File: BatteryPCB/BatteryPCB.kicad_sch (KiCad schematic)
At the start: 18 parts, among them J1 Conn_01x01, J2 Conn_01x01, J3 Conn_01x01, J4 Conn_01x01_Socket, SW1 ANT11TFHQE, SW3 ANT11TFHQE, U1 LF50CV, U2 R05-100B, U3 R05-100B

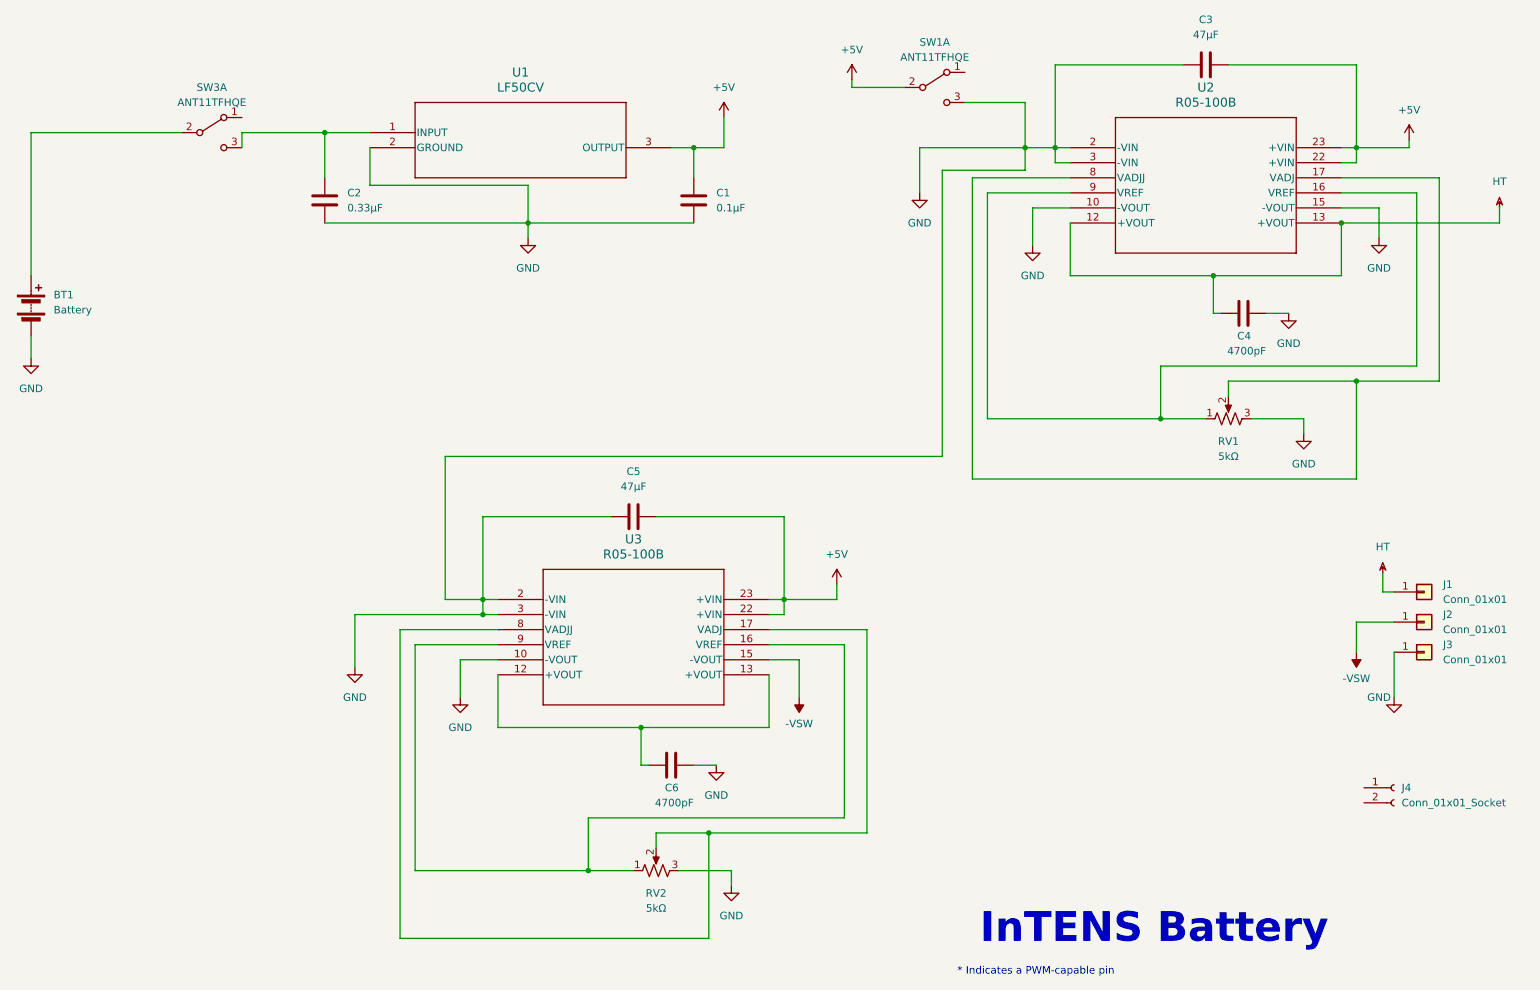
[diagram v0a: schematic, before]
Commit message: In progress changes from 3/29 2nd comments
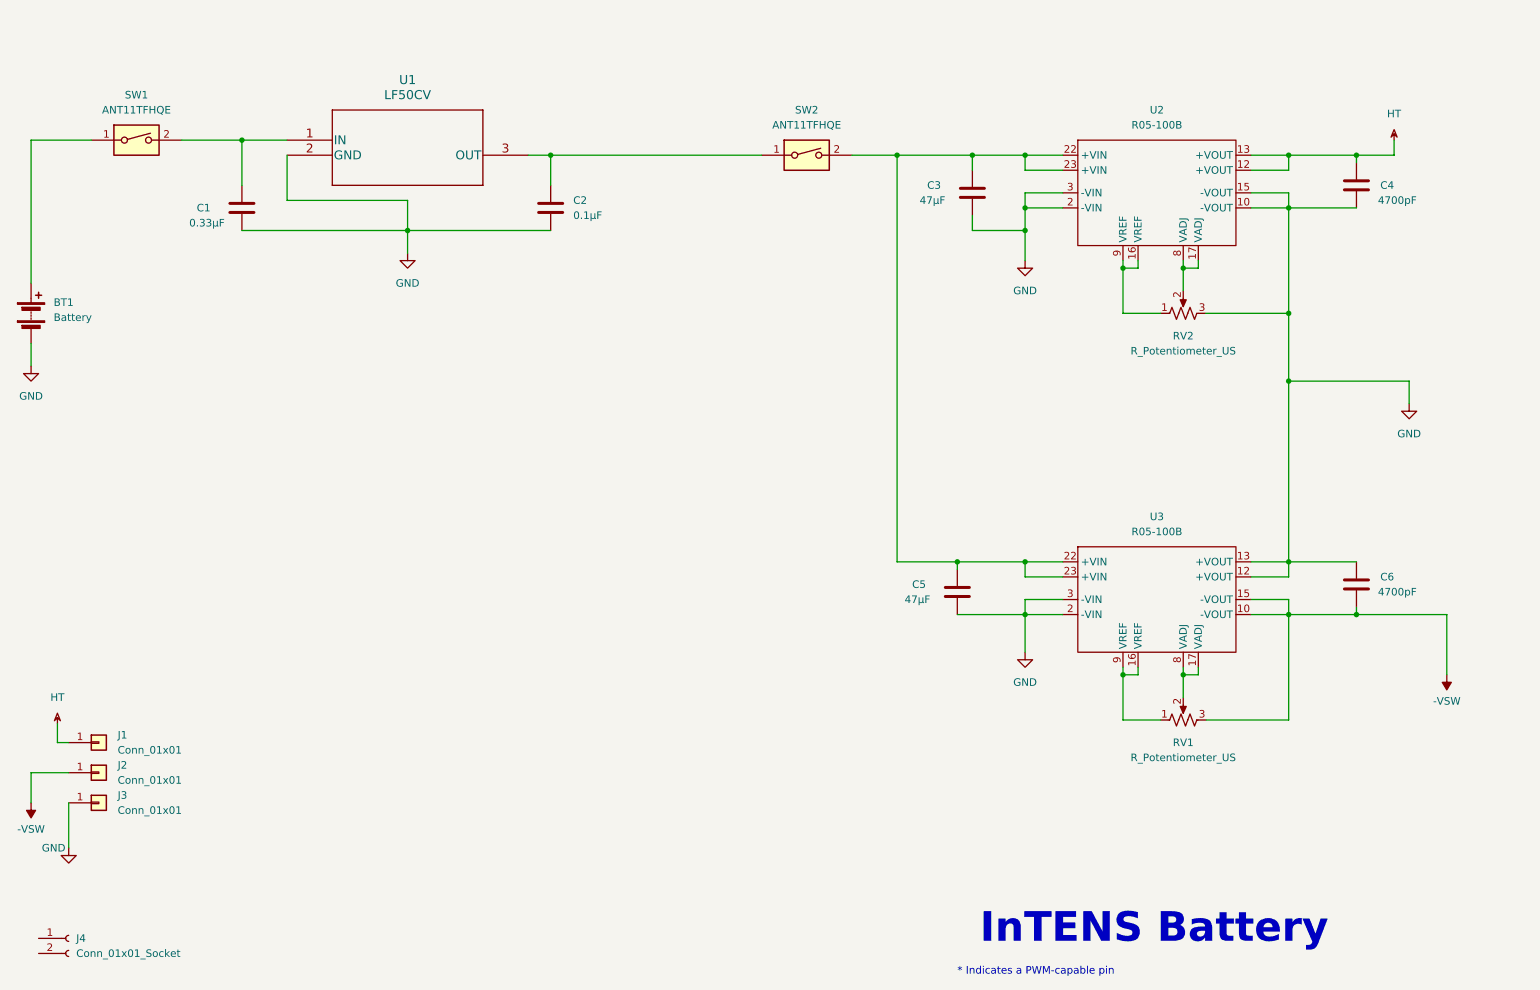
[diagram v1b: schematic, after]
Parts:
- removed SW1, SW3: ANT11TFHQE, 100SP1T1B4M2QE:100SP1T1_EWI, symbol Switch:SW_DPDT_x2
- removed U1: LF50CV, L7805CV:TO-220_STM, symbol L7805CV:L7805CV
- removed U2, U3: R05-100B, Package_DIP:DIP-24_W15.24mm, symbol R05_100B:R05-100B
- added SW1, SW2: ANT11TFHQE, 100SP1T1B4M2QE:100SP1T1_EWI, symbol Switch:SW_DIP_x01
- added U1: LF50CV, TO-220_STM, symbol LF50CV:LF50CV
- added U2, U3: R05-100B, Package_DIP:DIP-24_W15.24mm, symbol InTENS_customparts:R05-100B
- RV1, RV2: value 5kΩ -> R_Potentiometer_US; footprint Potentiometer_THT:Potentiometer_ACP_CA6-H2,5_Horizontal -> (none)
- renumbered C2 to C1, C1 to C2
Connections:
- net -VSW: now also C6.1, RV1.3, U3.10 (-VOUT), U3.15 (-VOUT)
- net GND: now also C4.1, U1.2 (GND), U2.10 (-VOUT), U2.15 (-VOUT), U2.2 (-VIN), U2.3 (-VIN), U3.12 (+VOUT), U3.13 (+VOUT), U3.2 (-VIN), U3.3 (-VIN); no longer C4.2, RV1.3
- net HT: now also C4.2, U2.12 (+VOUT), U2.13 (+VOUT); no longer C4.1
- net at RV2.1: now also U2.16 (VREF), U2.9 (VREF)
- net at RV2.2: now also U2.17 (VADJ), U2.8 (VADJ)
- net at RV1.1: now also U3.16 (VREF), U3.9 (VREF)
- net at RV1.2: now also U3.17 (VADJ), U3.8 (VADJ)
- net at BT1.1 (+): now also SW1.1
- net at C1.1: now also SW1.2, U1.1 (IN)
- net +5V: no longer names the net of C3.2, C5.2
- net +5V: now also SW2.2, U2.22 (+VIN), U2.23 (+VIN), U3.22 (+VIN), U3.23 (+VIN); no longer C2.1
- new net: C2.1, SW2.1, U1.3 (OUT)
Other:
- moved on the sheet: BT1, C1, C2, C3, C4, C5, C6, J1, J2, J3, J4
